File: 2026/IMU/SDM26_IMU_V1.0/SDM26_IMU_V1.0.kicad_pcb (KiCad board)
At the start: 4 copper layers, 52 x 41 mm, 58 parts, among them IC1 ESP32-S3-WROOM-1-N8R8, IC2 ISM330DHCXTR, IC3 CP2102N-A02-GQFN28, IC4 TPS259250DRCR, IC5 MIC37100-3.3WS, IC6 TPS2116DRLR, IC7 TLP175A_TPL,E, J1 Conn_01x04_Socket, J2 USB_B_Micro, Q1 MMBT2222LT1G, Q2 MMBT2222LT1G, U1 USBLC6-2SC6, U2 SN65HVD230

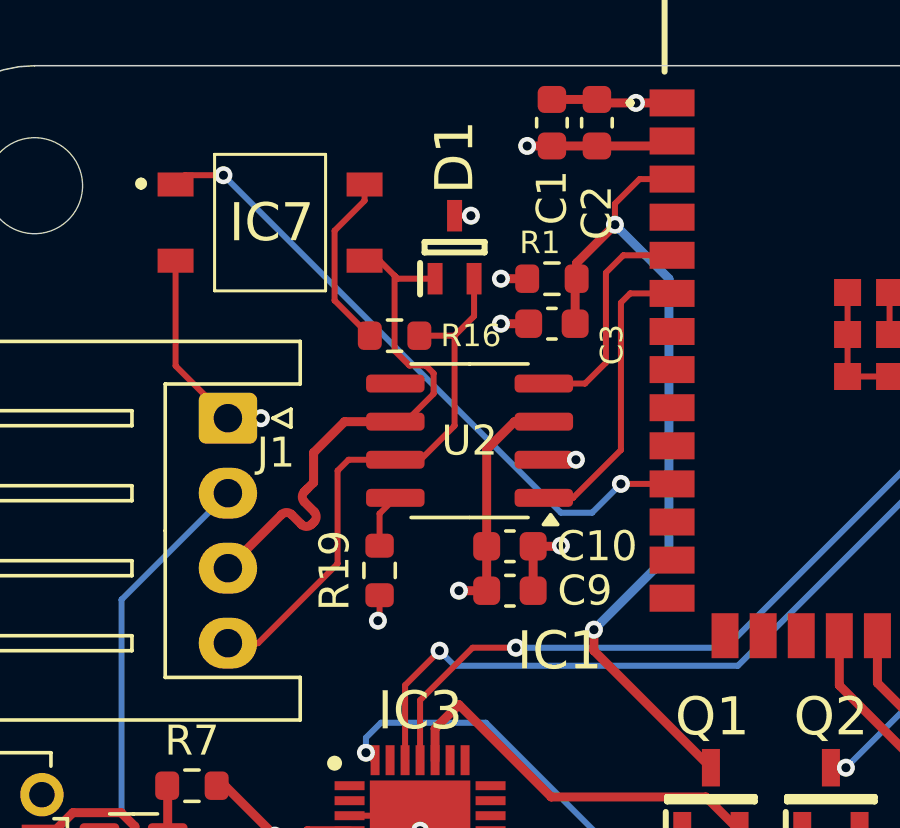
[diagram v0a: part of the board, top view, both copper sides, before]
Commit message: September order sync
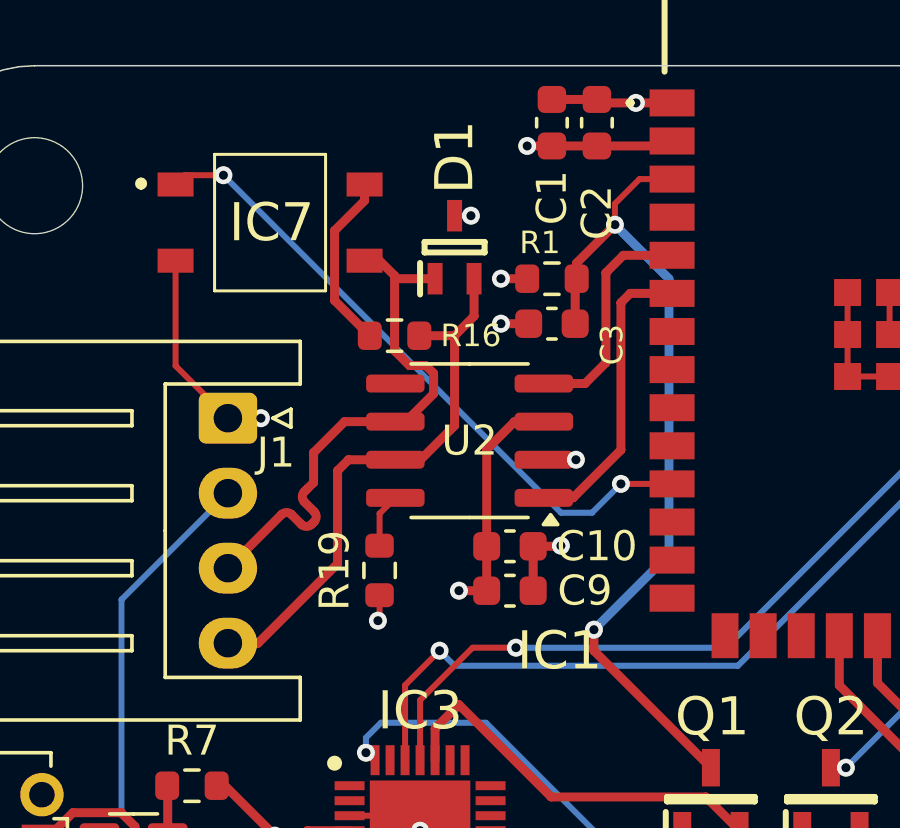
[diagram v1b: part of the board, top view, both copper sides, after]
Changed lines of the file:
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@@
 		(start 74.455 49.1)
 		(end 74.455 51.6)
-		(width 0.2)
+		(width 0.3)
 		(layer "F.Cu")
 		(net 4)
@@
 		(start 75.756 52.354032)
 		(end 75.756 53.035968)
-		(width 0.2)
+		(width 0.3)
 		(layer "F.Cu")
 		(net 4)
@@
 		(start 74.949 52.094)
 		(end 75.495968 52.094)
-		(width 0.2)
+		(width 0.3)
 		(layer "F.Cu")
 		(net 4)
@@
 		(start 74.826968 53.965)
 		(end 74.48 53.965)
-		(width 0.2)
+		(width 0.3)
 		(layer "F.Cu")
 		(net 4)
@@
 		(start 74.455 51.6)
 		(end 74.949 52.094)
-		(width 0.2)
+		(width 0.3)
 		(layer "F.Cu")
 		(net 4)
@@
 		(start 73.955 48.6)
 		(end 74.455 49.1)
-		(width 0.2)
+		(width 0.3)
 		(layer "F.Cu")
 		(net 4)
@@
 		(start 75.756 53.035968)
 		(end 74.826968 53.965)
-		(width 0.2)
+		(width 0.3)
 		(layer "F.Cu")
 		(net 4)
@@
 		(start 75.495968 52.094)
 		(end 75.756 52.354032)
-		(width 0.2)
+		(width 0.3)
 		(layer "F.Cu")
 		(net 4)
@@
 		(start 75.805 49.2)
 		(end 74.555 49.2)
-		(width 0.2)
+		(width 0.3)
 		(layer "F.Cu")
 		(net 4)
@@
 		(start 69.905 61.35)
 		(end 72.555 58.7)
-		(width 0.2)
+		(width 0.3)
 		(layer "F.Cu")
 		(net 5)
@@
 		(start 72.555 55.6)
 		(end 72.92 55.235)
-		(width 0.2)
+		(width 0.3)
 		(layer "F.Cu")
 		(net 5)
@@
 		(start 77.105 50.45)
 		(end 77.105 49.2)
-		(width 0.2)
+		(width 0.3)
 		(layer "F.Cu")
 		(net 5)
@@
 		(start 76.455 51.1)
 		(end 77.105 50.45)
-		(width 0.2)
+		(width 0.3)
 		(layer "F.Cu")
 		(net 5)
@@
 		(start 76.455 51.1)
 		(end 76.455 54.1)
-		(width 0.2)
+		(width 0.3)
 		(layer "F.Cu")
 		(net 5)
@@
 		(start 72.555 58.7)
 		(end 72.555 55.6)
-		(width 0.2)
+		(width 0.3)
 		(layer "F.Cu")
 		(net 5)
@@
 		(start 75.28 51.1)
 		(end 76.455 51.1)
-		(width 0.2)
+		(width 0.3)
 		(layer "F.Cu")
 		(net 5)
@@
 		(start 72.92 55.235)
 		(end 74.48 55.235)
-		(width 0.2)
+		(width 0.3)
 		(layer "F.Cu")
 		(net 5)
@@
 		(start 75.32 55.235)
 		(end 74.48 55.235)
-		(width 0.2)
+		(width 0.3)
 		(layer "F.Cu")
 		(net 5)
@@
 		(start 68.9 61.35)
 		(end 69.905 61.35)
-		(width 0.2)
+		(width 0.3)
 		(layer "F.Cu")
 		(net 5)
@@
 		(start 76.455 54.1)
 		(end 75.32 55.235)
-		(width 0.2)
+		(width 0.3)
 		(layer "F.Cu")
 		(net 5)
@@
 		(start 81.5 52)
 		(end 81.5 49)
-		(width 0.2)
+		(width 0.3)
 		(layer "F.Cu")
 		(net 44)
@@
 		(start 82.08 48.42)
 		(end 83.705 48.42)
-		(width 0.2)
+		(width 0.3)
 		(layer "F.Cu")
 		(net 44)
@@
 		(start 79.43 52.695)
 		(end 80.805 52.695)
-		(width 0.2)
+		(width 0.3)
 		(layer "F.Cu")
 		(net 44)
@@
 		(start 80.805 52.695)
 		(end 81.5 52)
-		(width 0.2)
+		(width 0.3)
 		(layer "F.Cu")
 		(net 44)
@@
 		(start 81.5 49)
 		(end 82.08 48.42)
-		(width 0.2)
+		(width 0.3)
 		(layer "F.Cu")
 		(net 44)
@@
 		(start 82.31 49.69)
 		(end 83.705 49.69)
-		(width 0.2)
+		(width 0.3)
 		(layer "F.Cu")
 		(net 46)
@@
 		(start 82 54.909999)
 		(end 82 50)
-		(width 0.2)
+		(width 0.3)
 		(layer "F.Cu")
 		(net 46)
@@
 		(start 80.404999 56.505)
 		(end 82 54.909999)
-		(width 0.2)
+		(width 0.3)
 		(layer "F.Cu")
 		(net 46)
@@
 		(start 79.43 56.505)
 		(end 80.404999 56.505)
-		(width 0.2)
+		(width 0.3)
 		(layer "F.Cu")
 		(net 46)
@@
 		(start 82 50)
 		(end 82.31 49.69)
-		(width 0.2)
+		(width 0.3)
 		(layer "F.Cu")
 		(net 46)
@@
 		(start 72.455 49.925)
 		(end 72.455 47.6)
-		(width 0.2)
+		(width 0.3)
 		(layer "F.Cu")
 		(net 95)
@@
 		(start 72.455 47.6)
 		(end 73.455 46.6)
-		(width 0.2)
+		(width 0.3)
 		(layer "F.Cu")
 		(net 95)
@@
 		(start 73.455 46.6)
 		(end 73.455 46.06)
-		(width 0.2)
+		(width 0.3)
 		(layer "F.Cu")
 		(net 95)
@@
 		(start 73.63 51.1)
 		(end 72.455 49.925)
-		(width 0.2)
+		(width 0.3)
 		(layer "F.Cu")
 		(net 95)
